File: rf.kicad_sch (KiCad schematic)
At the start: 50 parts, among them IC1 SX1255IWLTRT, J1 Antenna, U7 GRF5604, U9 SKY13330-397LF, Y1 32MHz

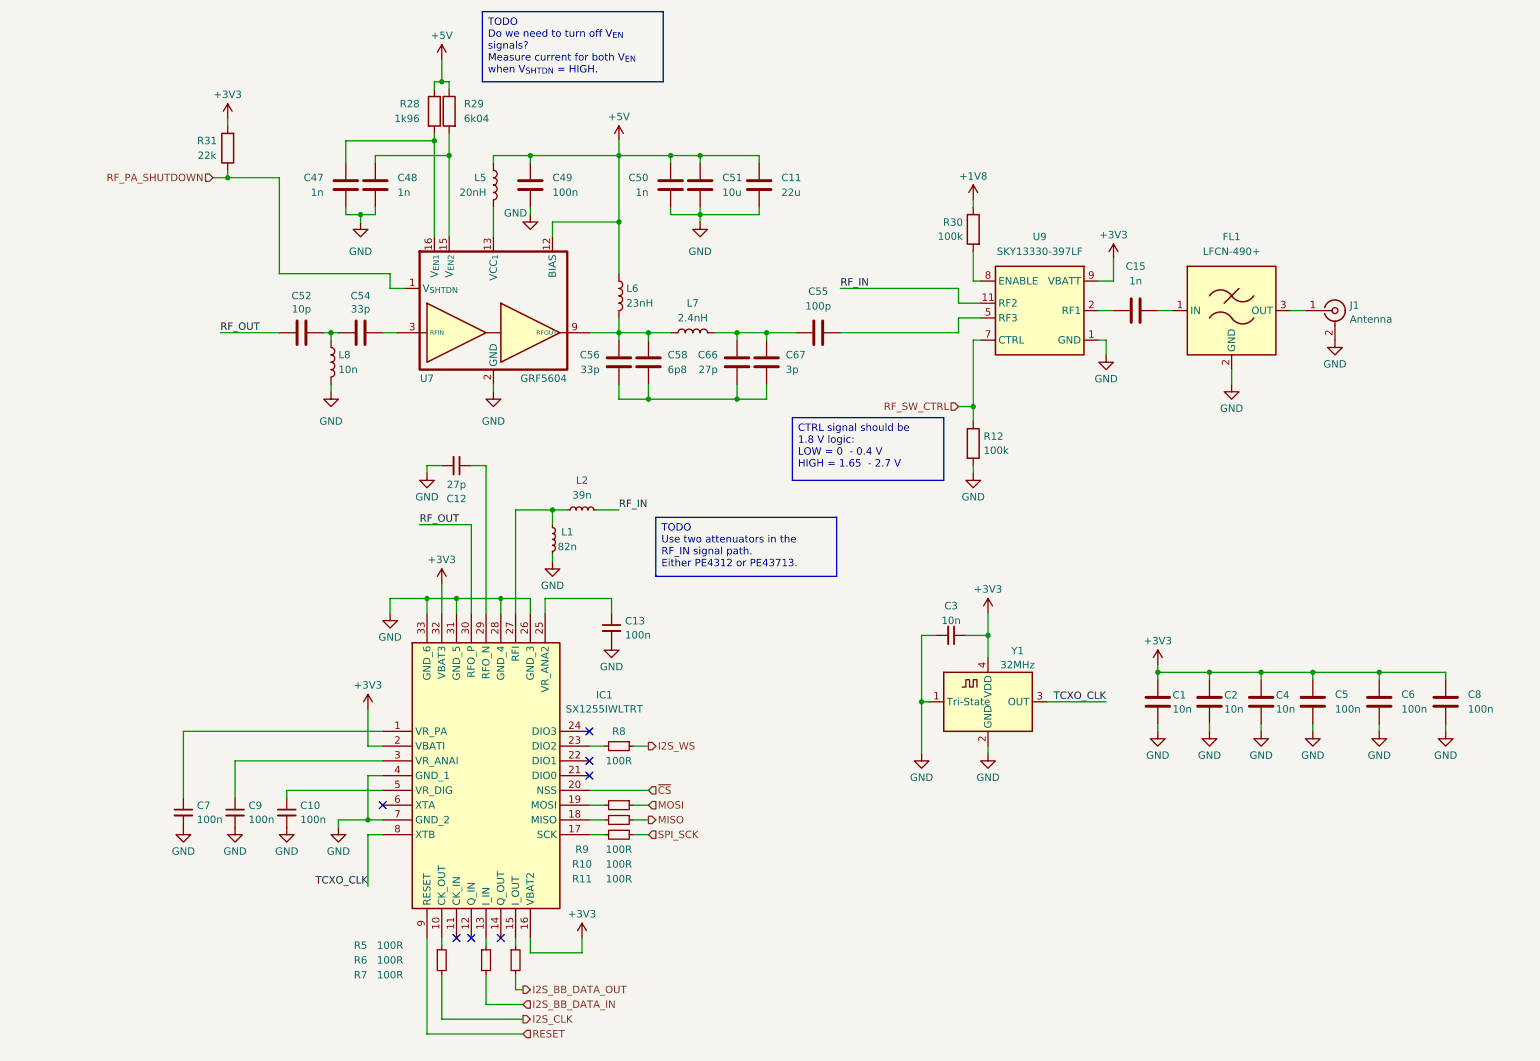
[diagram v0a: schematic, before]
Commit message: Added two series attenuators PE4312 to the RF input path
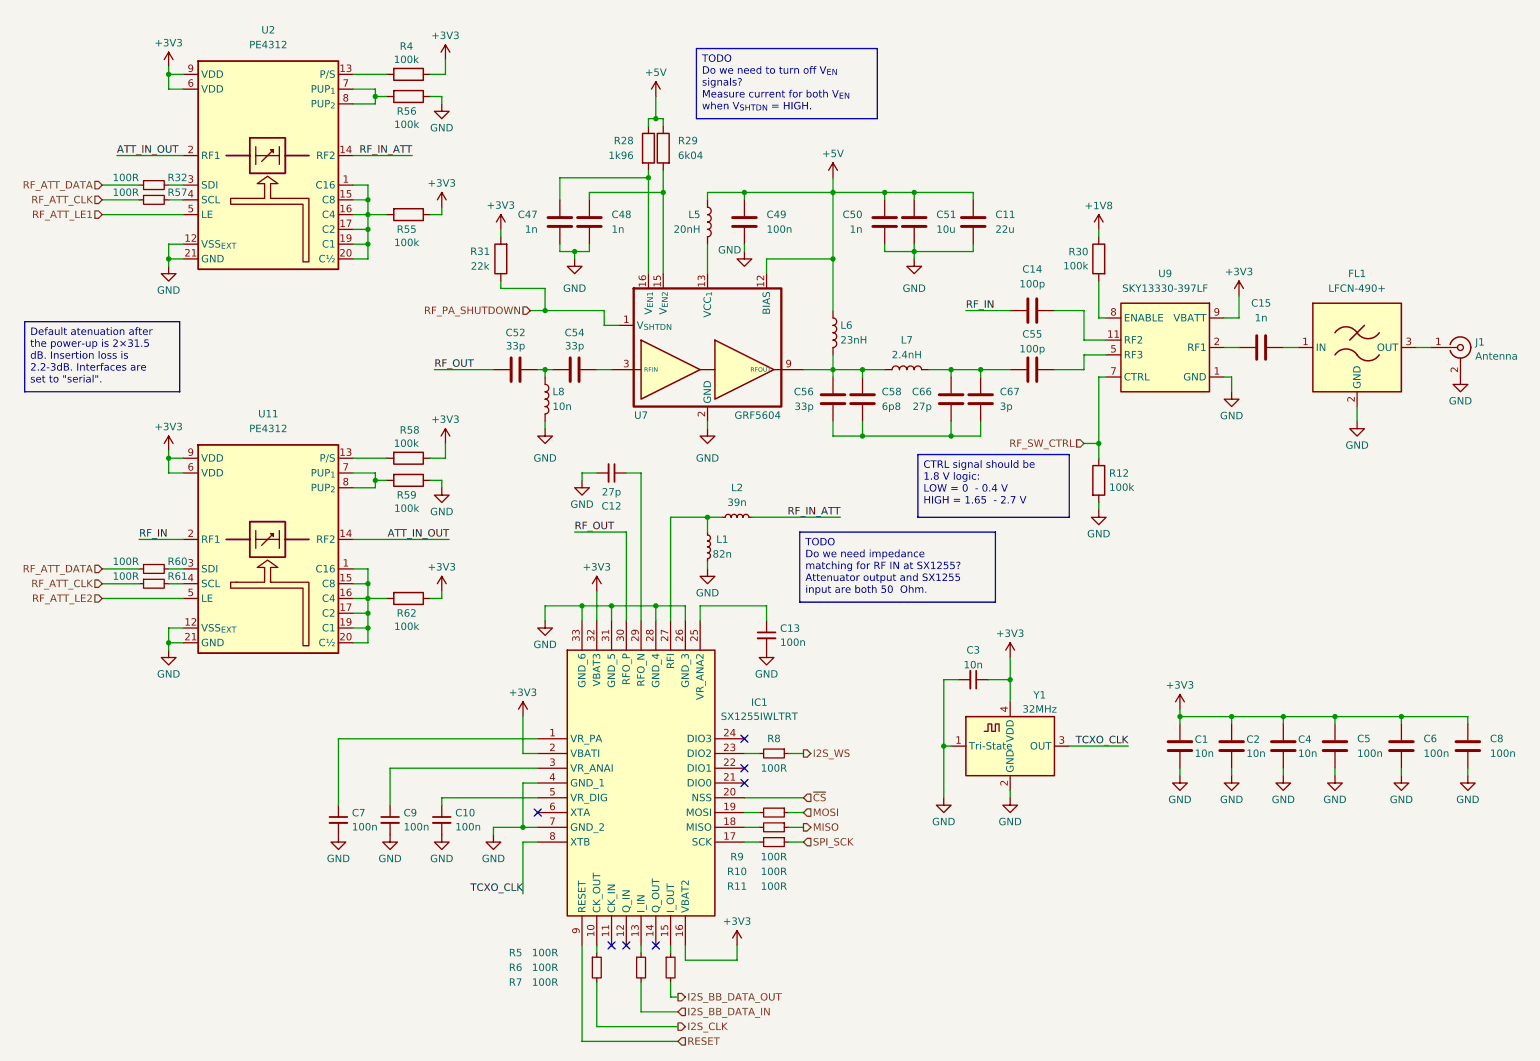
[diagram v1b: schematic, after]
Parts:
- added C14: 100p, Capacitor_SMD:C_0402_1005Metric, symbol Device:C
- added R32, R57, R60, R61: 100R, Resistor_SMD:R_0402_1005Metric, symbol Device:R_Small
- added R4, R55, R56, R58, R59, R62: 100k, Resistor_SMD:R_0402_1005Metric, symbol Device:R
- added U11, U2: PE4312, Package_DFN_QFN:QFN-20-1EP_4x4mm_P0.5mm_EP2.5x2.5mm, symbol parts:PE4312
- C52: value 10p -> 33p
- U7: MPN (none) -> GRF5604; PN (none) -> 459-GRF5604
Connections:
- net +3V3: now also R4.1, R55.1, R58.1, R62.1, U11.6 (VDD), U11.9 (VDD), U2.6 (VDD), U2.9 (VDD)
- net GND: now also R56.1, R59.1, U11.10 (GND), U11.11 (GND), U11.12 (VSS_{EXT}), U11.18 (GND), U11.21 (GND), U2.10 (GND), U2.11 (GND), U2.12 (VSS_{EXT}), U2.18 (GND), U2.21 (GND)
- net RF_IN: now also C14.1, U11.2 (RF1); no longer L2.1, U9.11 (RF2)
- new net: R4.2, U2.13 (P/S)
- new net: C14.2, U9.11 (RF2)
- new net: R62.2, U11.1 (C16), U11.15 (C8), U11.16 (C4), U11.17 (C2), U11.19 (C1), U11.20 (C½)
- new net: R58.2, U11.13 (P/S)
- new net: R60.2, U11.3 (SDI)
- new net: R61.2, U11.4 (SCL)
- new net: R59.2, U11.7 (PUP_{1}), U11.8 (PUP_{2})
- new net: R56.2, U2.7 (PUP_{1}), U2.8 (PUP_{2})
- new net: R57.2, U2.4 (SCL)
- new net: R55.2, U2.1 (C16), U2.15 (C8), U2.16 (C4), U2.17 (C2), U2.19 (C1), U2.20 (C½)
- new net: R32.2, U2.3 (SDI)
- new net ATT_IN_OUT: U11.14 (RF2), U2.2 (RF1)
- new net RF_ATT_CLK: R57.1, R61.1
- new net RF_ATT_DATA: R32.1, R60.1
- new net RF_ATT_LE1: U2.5 (LE)
- new net RF_ATT_LE2: U11.5 (LE)
- new net RF_IN_ATT: L2.1, U2.14 (RF2)
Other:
- moved on the sheet: C1, C10, C11, C12, C13, C15, C2, C3, C4, C47, C48, C49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

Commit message: Fixed and added LCSC reference numbers for all components
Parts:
- C14, C55: MPN (none) -> GRM1555C1H101JA01D
- C47, C48, C50: LCSC C161523 -> C113780; MPN (none) -> CC0402JRNPO9BN102; PN (none) -> 603-CC402JRNPO9BN102
- C49: LCSC C913614 -> C1525; MPN (none) -> CL05B104KO5NNNC; PN (none) -> 187-CL05B104KO5NNNC
- C51: LCSC C237279 -> C15525; MPN (none) -> CL05A106MQ5NUNC; PN (none) -> 187-CL05A106MQ5NUNC
- C52: LCSC C782046 -> C464434; MPN (none) -> GJM1555C1H330FB01D
- C54, C56: MPN (none) -> GJM1555C1H330FB01D
- C66: LCSC C88883 -> C107002; MPN (none) -> CC0402JRNPO9BN270; PN (none) -> 603-CC402JRNPO9BN270
- R10, R11, R32, R5, R57, R6, R60, R61, R7, R8, R9: MPN (none) -> 0402WGF1000TCE; PN 0402WGF1000TCE -> (none)
- R12, R30, R4, R55, R56, R58, R59, R62: MPN (none) -> 0402WGF1003TCE; PN 0402WGF1003TCE -> (none)
- R31: MPN (none) -> 0402WGF2202TCE; PN 0402WGF2202TCE -> (none)
- U7: footprint Parts:QFN-16-1EP_3x3mm_P0.5mm_EP1.7x1.7mm_ThermalVias -> parts:QFN-16-1EP_3x3mm_P0.5mm_EP1.7x1.7mm_ThermalVias; LCSC (none) -> GRF5604
- U9: LCSC (none) -> C2654715; MPN (none) -> SKY13330-397LF
- Y1: footprint Crystal:Crystal_SMD_2016-4Pin_2.0x1.6mm -> Oscillator:Oscillator_SMD_ECS_2520MV-xxx-xx-4Pin_2.5x2.0mm

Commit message: Fixed oscillator footprints
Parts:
- Y1: footprint Oscillator:Oscillator_SMD_ECS_2520MV-xxx-xx-4Pin_2.5x2.0mm -> Crystal:Crystal_SMD_2016-4Pin_2.0x1.6mm
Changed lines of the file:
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@@
 			)
 		)
-		(property "Footprint" "Oscillator:Oscillator_SMD_ECS_2520MV-xxx-xx-4Pin_2.5x2.0mm"
+		(property "Footprint" "Crystal:Crystal_SMD_2016-4Pin_2.0x1.6mm"
 			(at 204.47 151.13 0)
 			(effects
